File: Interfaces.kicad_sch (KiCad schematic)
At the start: 4 parts, among them J1 1-84952-0, J2 1-84952-0, U10 USBLC6-2SC6

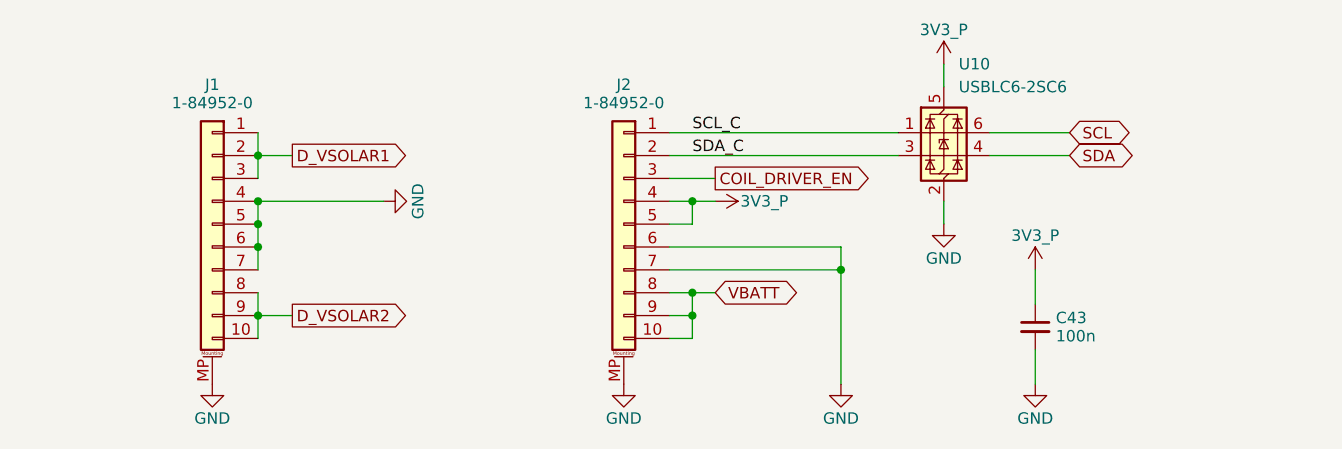
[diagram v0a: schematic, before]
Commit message: Local Stash
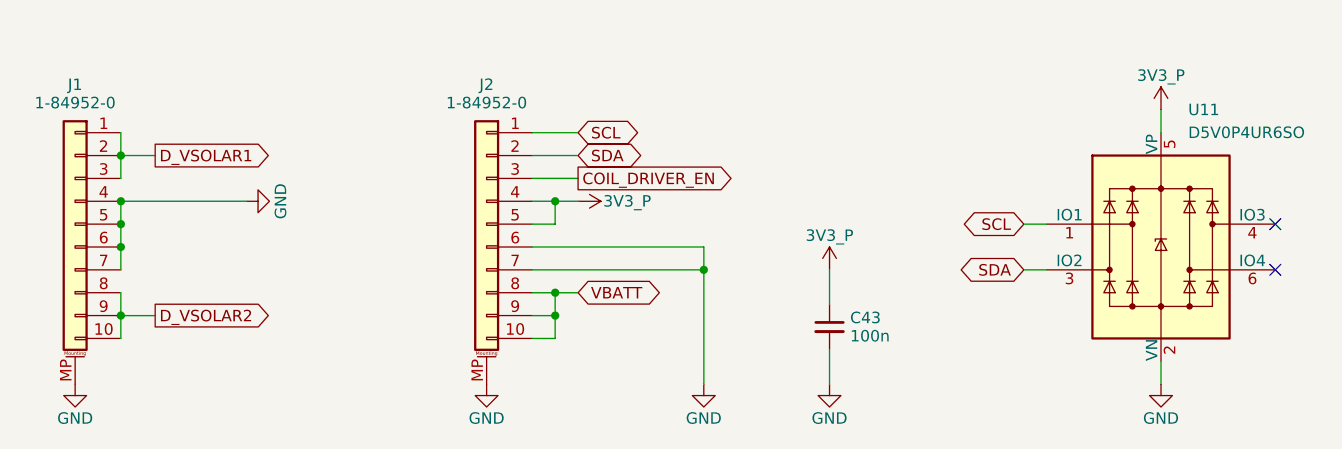
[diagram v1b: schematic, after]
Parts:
- removed U10: USBLC6-2SC6, Package_TO_SOT_SMD:SOT-23-6, symbol Power_Protection:USBLC6-2SC6
- added U11: D5V0P4UR6SO, Package_TO_SOT_SMD:SOT-23-6, symbol Power_Protection:SRV05-4
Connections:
- net SCL_C is gone; now on net SCL: J2.1 (Pin_1)
- net SDA_C is gone; now on net SDA: J2.2 (Pin_2)
- net 3V3_P: now also U11.5 (VP)
- net GND: now also U11.2 (VN)
- net SCL: now also U11.1 (IO1)
- net SDA: now also U11.3 (IO2)
- no-connect marks 0 -> 2
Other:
- moved on the sheet: C43, J1, J2
